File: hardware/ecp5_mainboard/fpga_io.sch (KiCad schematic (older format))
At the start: 75 parts, among them J10 UART, J11 FLASH, J12 JTAG, J5 EXT0, J6 EXT1, J7 EXT2, J8 EXT3, J9 PMOD_01, Q9 BSH111BKR, SW6 SW_Push, U15 ECP5UM5G_85_CABGA756, U26 XL_XO_LVDS, U27 W25Q

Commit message: hardware/mainboard: All parts placed
Signed-off-by: David Shah <dave@ds0.me>
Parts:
- J11: footprint Connector_PinHeader_2.54mm:PinHeader_1x08_P2.54mm_Vertical -> Connector_PinHeader_2.54mm:PinHeader_2x04_P2.54mm_Vertical
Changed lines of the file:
@@
 F 0 "J11" H 19150 10667 50  0000 C CNN
 F 1 "FLASH" H 19150 10576 50  0000 C CNN
-F 2 "Connector_PinHeader_2.54mm:PinHeader_1x08_P2.54mm_Vertical" H 19100 10350 50  0001 C CNN
+F 2 "Connector_PinHeader_2.54mm:PinHeader_2x04_P2.54mm_Vertical" H 19100 10350 50  0001 C CNN
 F 3 "~" H 19100 10350 50  0001 C CNN
 	1    19100 10350

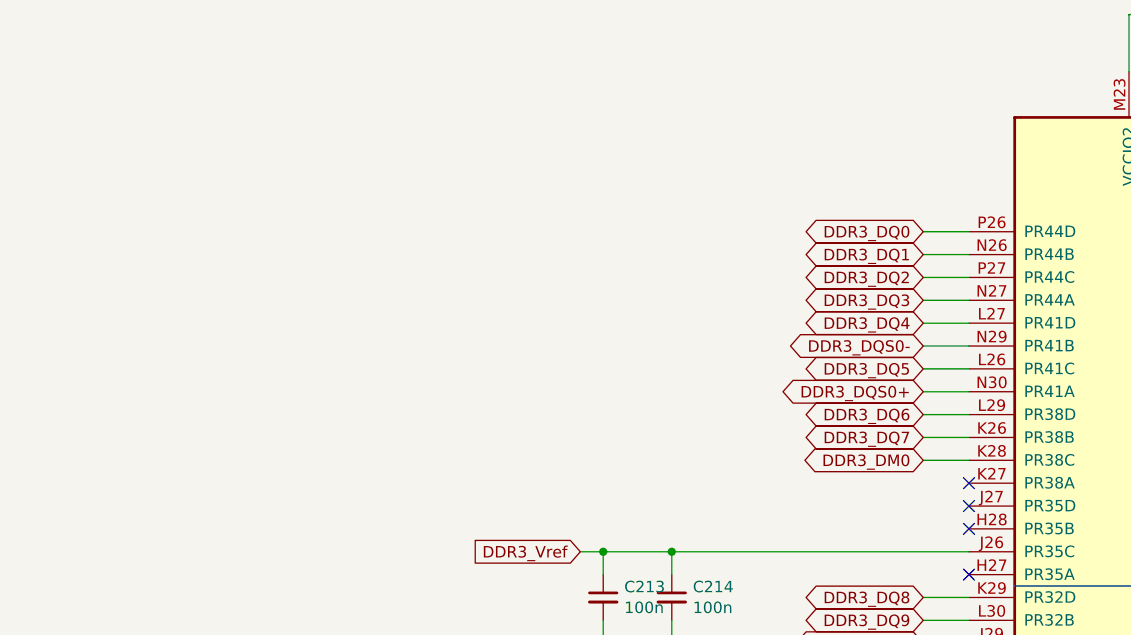
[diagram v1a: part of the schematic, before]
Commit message: hardware/mainboard: Tidying up
Signed-off-by: David Shah <dave@ds0.me>
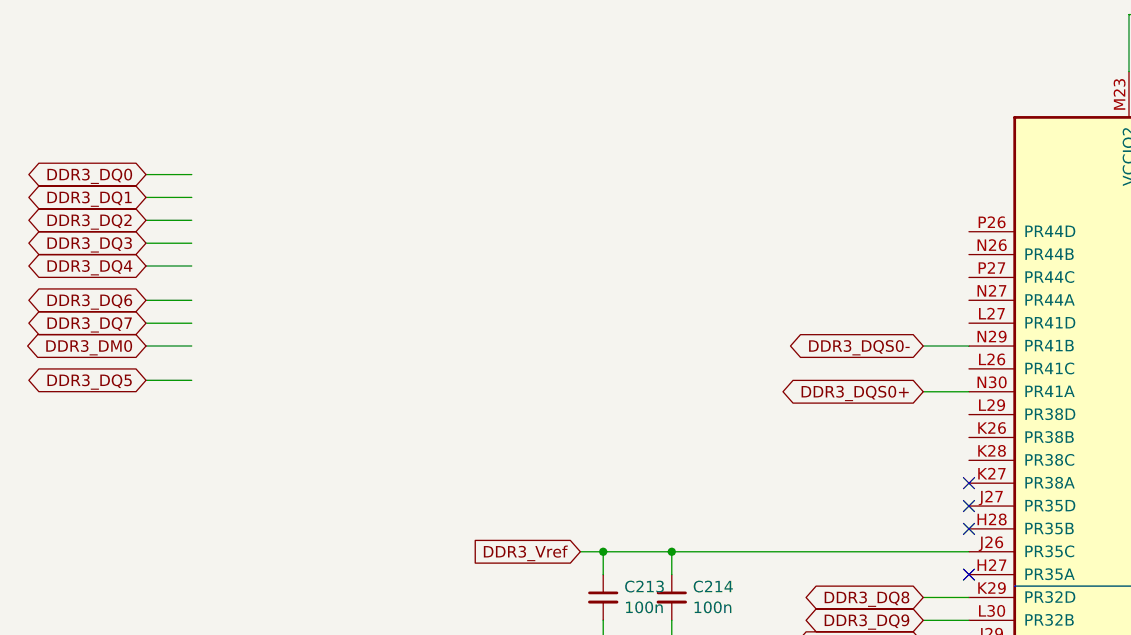
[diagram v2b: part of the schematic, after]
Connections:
- net DDR3_DM0: no longer U15.K28 (PR38C)
- net DDR3_DQ0: no longer U15.P26 (PR44D)
- net DDR3_DQ1: no longer U15.N26 (PR44B)
- net DDR3_DQ2: no longer U15.P27 (PR44C)
- net DDR3_DQ3: no longer U15.N27 (PR44A)
- net DDR3_DQ4: no longer U15.L27 (PR41D)
- net DDR3_DQ5: no longer U15.L26 (PR41C)
- net DDR3_DQ6: no longer U15.L29 (PR38D)
- net DDR3_DQ7: no longer U15.K26 (PR38B)
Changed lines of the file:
@@
 Text GLabel 2150 2450 0    50   BiDi ~ 0
 DDR3_DQS0-
-Text GLabel 2150 1950 0    50   BiDi ~ 0
+Text GLabel -1250 1700 0    50   BiDi ~ 0
 DDR3_DQ0
-Text GLabel 2150 2050 0    50   BiDi ~ 0
+Text GLabel -1250 1800 0    50   BiDi ~ 0
 DDR3_DQ1
-Text GLabel 2150 2150 0    50   BiDi ~ 0
+Text GLabel -1250 1900 0    50   BiDi ~ 0
 DDR3_DQ2
-Text GLabel 2150 2250 0    50   BiDi ~ 0
+Text GLabel -1250 2000 0    50   BiDi ~ 0
 DDR3_DQ3
-Text GLabel 2150 2350 0    50   BiDi ~ 0
+Text GLabel -1250 2100 0    50   BiDi ~ 0
 DDR3_DQ4
-Text GLabel 2150 2550 0    50   BiDi ~ 0
+Text GLabel -1250 2600 0    50   BiDi ~ 0
 DDR3_DQ5
-Text GLabel 2150 2750 0    50   BiDi ~ 0
+Text GLabel -1250 2250 0    50   BiDi ~ 0
 DDR3_DQ6
-Text GLabel 2150 2850 0    50   BiDi ~ 0
+Text GLabel -1250 2350 0    50   BiDi ~ 0
 DDR3_DQ7
-Text GLabel 2150 2950 0    50   BiDi ~ 0
+Text GLabel -1250 2450 0    50   BiDi ~ 0
 DDR3_DM0
 Wire Wire Line
-	2150 1950 2350 1950
+	-1250 1700 -1050 1700
 Wire Wire Line
-	2150 2050 2350 2050
+	-1250 1800 -1050 1800
 Wire Wire Line
-	2150 2150 2350 2150
+	-1250 1900 -1050 1900
 Wire Wire Line
-	2150 2250 2350 2250
+	-1250 2000 -1050 2000
 Wire Wire Line
-	2150 2350 2350 2350
+	-1250 2100 -1050 2100
 Wire Wire Line
 	2150 2450 2350 2450
 Wire Wire Line
-	2150 2550 2350 2550
+	-1250 2600 -1050 2600
 Wire Wire Line
 	2150 2650 2350 2650
 Wire Wire Line
-	2150 2750 2350 2750
+	-1250 2250 -1050 2250
 Wire Wire Line
-	2150 2850 2350 2850
+	-1250 2350 -1050 2350
 Wire Wire Line
-	2150 2950 2350 2950
+	-1250 2450 -1050 2450
 Text GLabel 5400 1900 0    50   Input ~ 0
 DIP_SW0
